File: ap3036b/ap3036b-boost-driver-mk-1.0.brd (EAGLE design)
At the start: 24 x 20 mm, 14 parts, among them IC1 ATTiny13, IC2 AMC7135

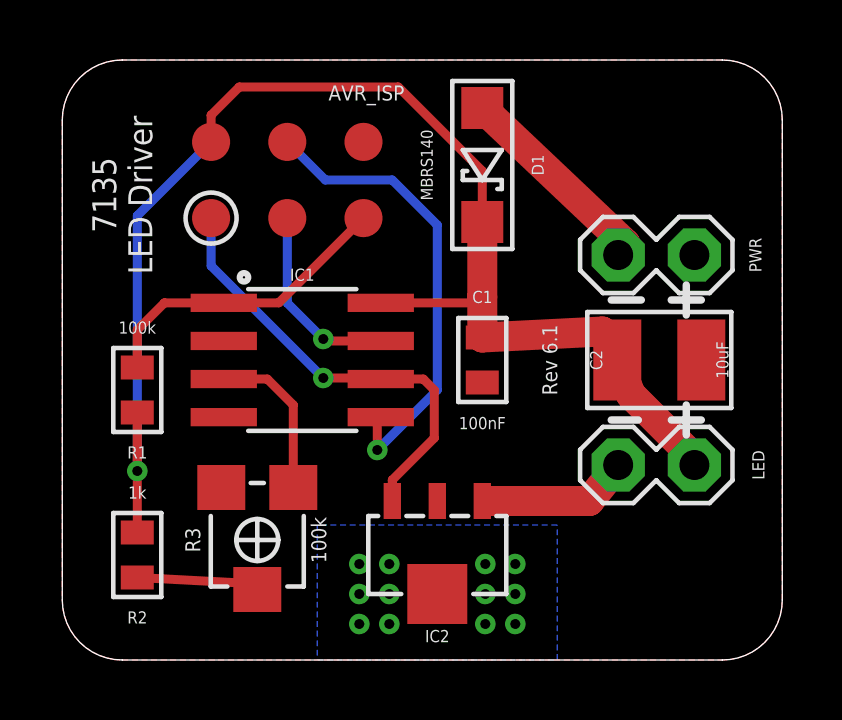
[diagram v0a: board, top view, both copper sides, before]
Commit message: whoa nelly lots of boards never quite finished
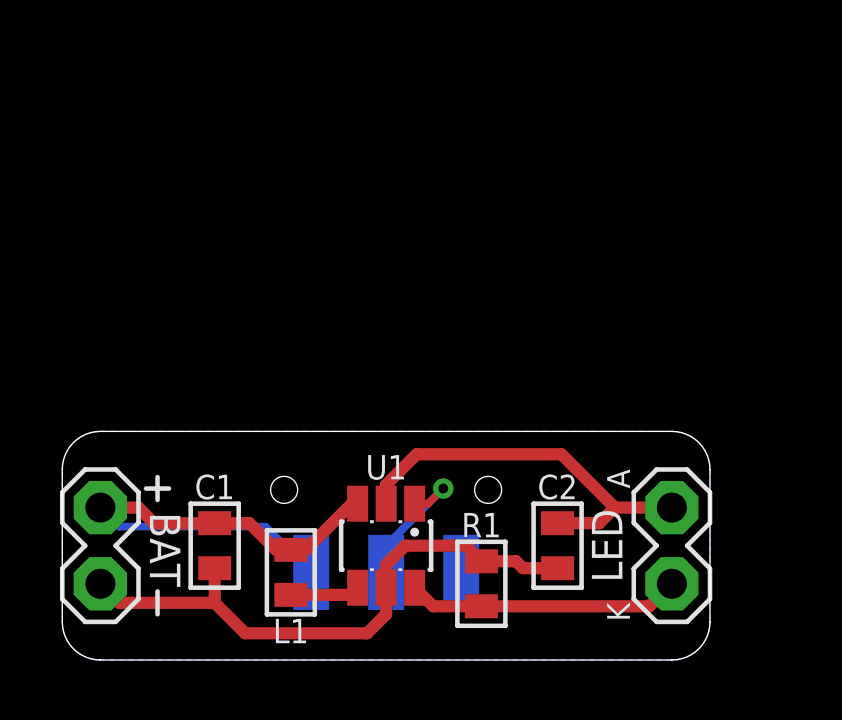
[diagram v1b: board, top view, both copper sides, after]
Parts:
- removed AVR_ISP: AVR_SPI_PRG_6SMD_TEST_POINTS, a_parts:2X3_SMD_TEST_POINTS
- removed D1: MBRS140, a_parts:SOD123-SCHOTTKY
- removed IC1: ATTiny13, a_parts:SO08
- removed IC2: AMC7135, a_parts:SOT89-NOTHERM
- removed PWR: M02PTH-CENTERED, a_parts:1X02-CENTER
- removed R2: 1k, a_parts:R0603-TIGHTER
- removed R3: 100k, A_butts:EVM3Y
- removed U$1: (no value), A_butts:CC-BY-SA-4.0-NO-URL
- removed U$2: (no value), A_butts:COW_SMALL
- added BAT: M02PTH-CENTERED, a_parts:1X02-CENTER
- added L1: 22uH, a_parts:L0603
- added S1: SWITCH-SPDTJS102011SAQN, a_parts:SWITCH-SPDT-SMD-RA-JS102011SAQN
- added U1: AP3036B, a_parts:SOT26
- C1: value 100nF -> 1uF
- C2: value 10uF -> 0.22uF; device a_parts:C1210 -> a_parts:C0603-TIGHTER
- R1: value 100k -> 10R
- moved R1 13.2 mm to (14.0, 2.54), turned to 270 degrees
- moved C1 10.9 mm to (5.08, 3.81)
- moved C2 7.06 mm to (16.5, 3.81), turned to 270 degrees
- moved LED 2.74 mm to (20.3, 3.81), turned to 90 degrees
- moved FRAME1 0.71 mm to (0.00, 0.00)
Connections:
- removed net BRIGHTNESS: IC1.3, R3.A
- removed net LED-: IC2.1, LED.2
- removed net MOSI: AVR_ISP.4, IC1.5
- removed net N$1: R2.1, R3.S
- removed net PWM: AVR_ISP.1, IC1.6, IC2.3
- removed net RST: AVR_ISP.5, IC1.1, R1.2
- removed net SCK: AVR_ISP.3, IC1.7
- removed net VCC: AVR_ISP.2, C1.1, C2.1, D1.C, IC1.8, LED.1, R1.1, R2.2
- new net LED_A: C2.1, LED.2, U1.2
- new net LED_K: LED.1, R1.2, U1.6
- new net SW: L1.2, U1.4
- new net VIN: BAT.2, C1.1, L1.1, S1.1, U1.3
- net GND: now also BAT.1, R1.1, S1.3, U1.5; no longer AVR_ISP.6, IC1.4, IC2.4@1, IC2.4@2, PWR.2, R3.E
- net N$2: now also S1.2, U1.1; no longer D1.A, PWR.1
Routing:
- net VCC: track 46.0 -> 0.00 mm, vias 1 -> 0
- net GND: track 0.00 -> 19.6 mm, vias 12 -> 0
- net VIN: track 0.00 -> 17.7 mm
- net MOSI: track 15.6 -> 0.00 mm, vias 1 -> 0
- net PWM: track 15.0 -> 0.00 mm, vias 1 -> 0
- net LED_A: track 0.00 -> 13.4 mm
- net RST: track 10.3 -> 0.00 mm
- net LED_K: track 0.00 -> 9.14 mm
- net SCK: track 6.47 -> 0.00 mm, vias 1 -> 0
- net BRIGHTNESS: track 5.42 -> 0.00 mm
- net LED-: track 5.11 -> 0.00 mm
- net N$1: track 4.09 -> 0.00 mm
- net SW: track 0.00 -> 2.32 mm
- net N$2: track 7.02 -> 4.75 mm, vias 0 -> 1
- removed copper zone on layer 1, net GND
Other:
- board size 24 x 20 mm -> 21.6 x 7.6 mm
- board text added: ">VERSION"
- board text added: "A"
- board text added: "Boost"
- board text added: "K"
- board text added: "LED Driver"
- board text removed: "7135 LED Driver"
- board text removed: ">REVISION"
- board text removed: "by schizobovine <sean@yak.net>"
